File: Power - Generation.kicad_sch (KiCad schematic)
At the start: 38 parts, among them U3 TPSM63603RDHR, U4 TPS62162DSG, U5 TLV75533PDBVR

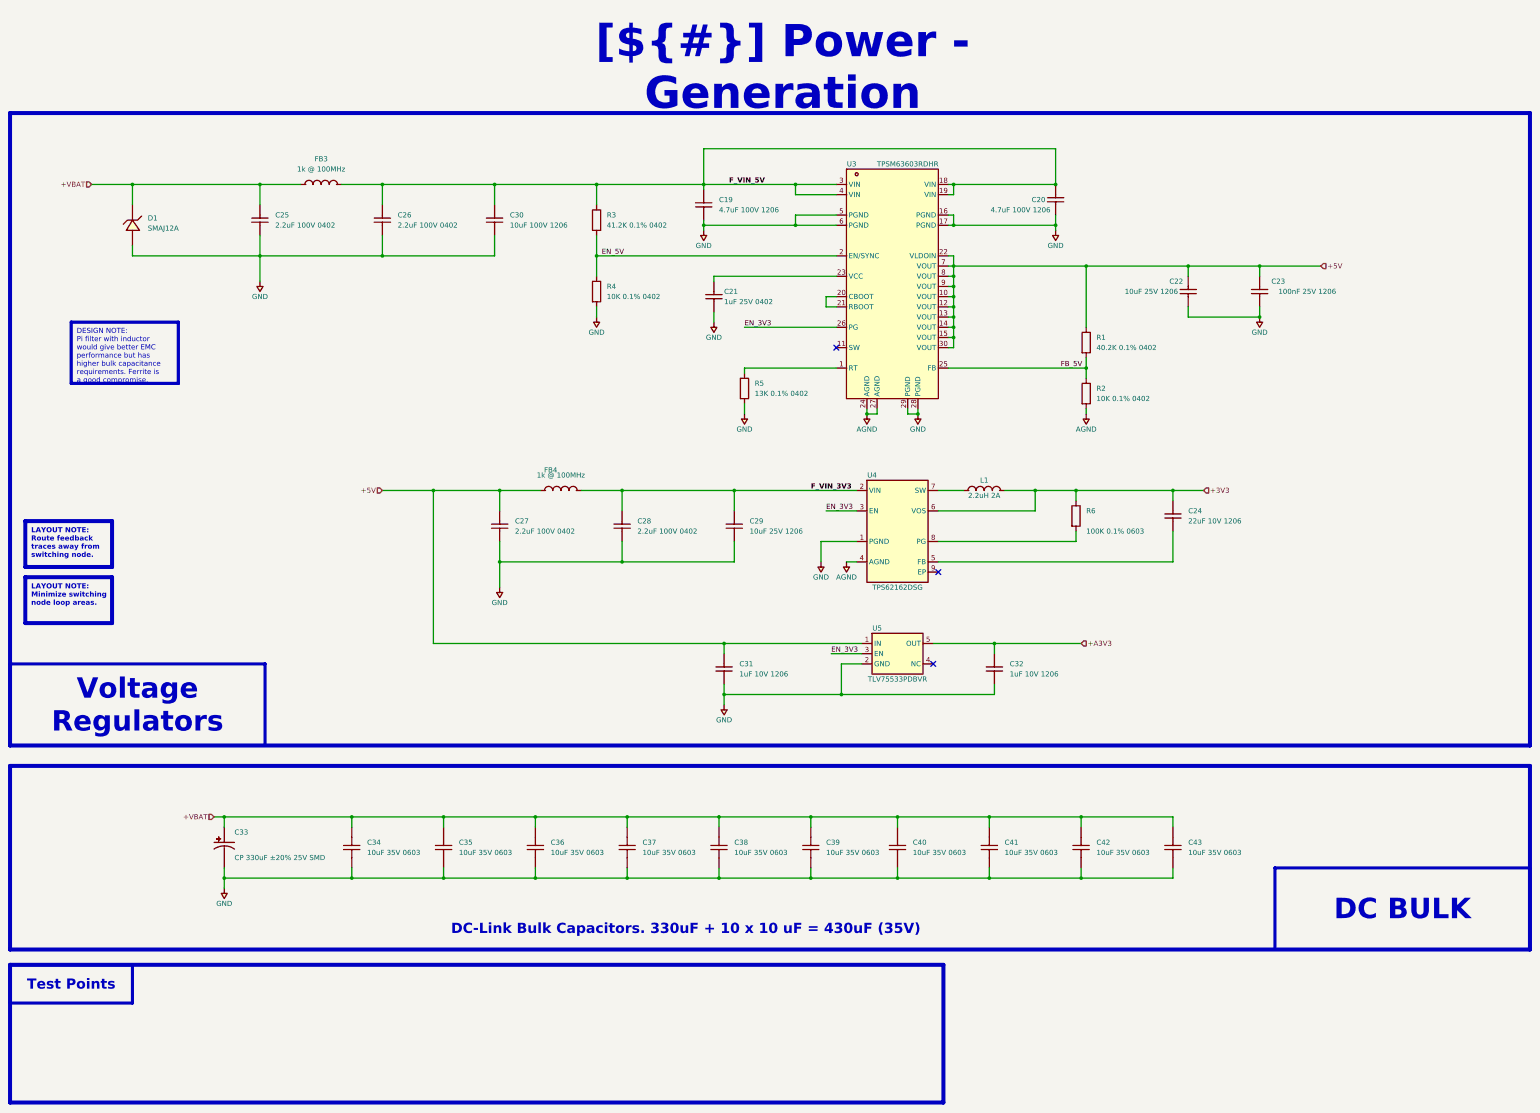
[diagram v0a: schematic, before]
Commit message: Update Schematic
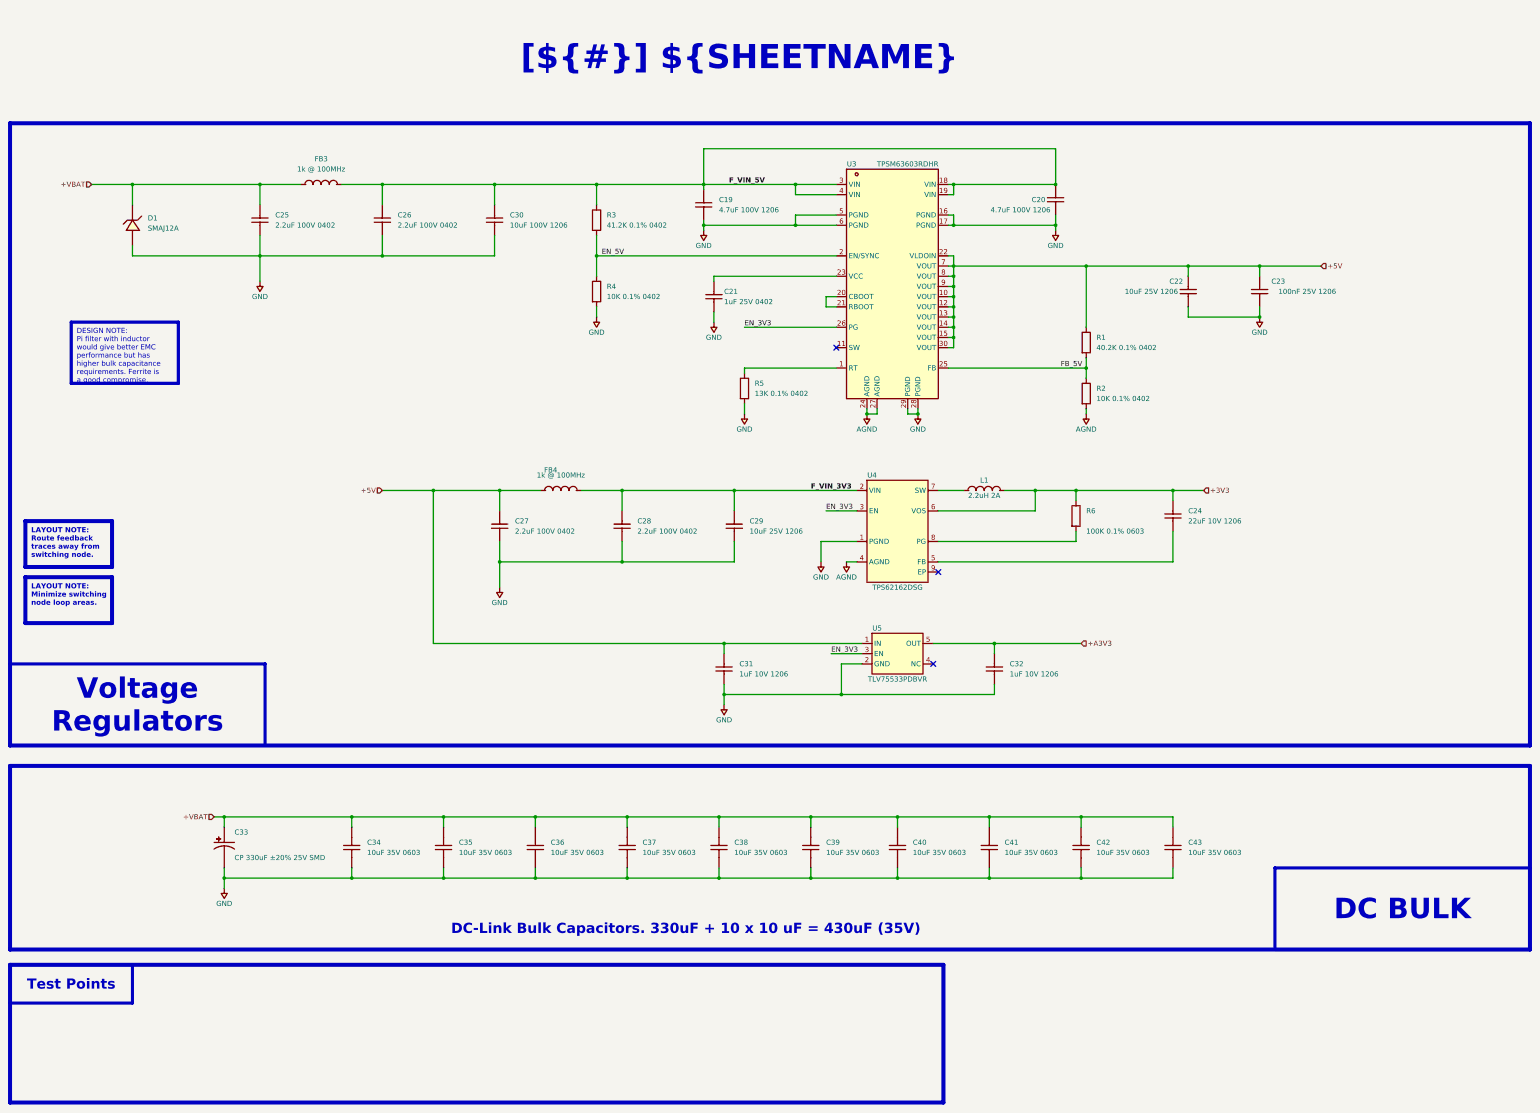
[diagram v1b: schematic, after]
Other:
- title: Power - Generation -> (none)
